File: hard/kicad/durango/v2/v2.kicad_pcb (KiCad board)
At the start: 2 copper layers, 177.8 x 130.8 mm, 155 parts, among them J1 NANOLINK, J10 STEP, J11 EXPANSION, J2 AUDIO IN, J3 IOx, J4 LED, J605 COMPONENT VIDEO, J7 POWER IN, J706 COMPOSITE, J8 DEBUG, J9 CARTRIDGE, J905 SCART, Q1 BC548, Q2 BC548, Q3 BC548, Q307 BC548, Q4 BC548, Q5 BC548, Q608 BC548, Q609 BC548, Q610 BC548, Q611 BC548, Q906 BC548, SW1 RESET, SW2 NMI, U1 65C02, U10 74HC139, U104 74HC257, U105 74HC257, U11 74HC688, U12 74HC74, U124 74HC574, U125 74HC157, U126 74HC86, U127 74HC245, U13 74HC32, U14 74HC4040, U15 74HC4040, U16 74HC02, U17 74HC21, U18 74HC85, U19 CD4040, U20 74HC85, U204 74HC257, U205 74HC257, U22 74HC175, U224 74HC166, U227 74HC20, U23 74HC86, U29 74HC139, U3 62256, U31 74HC245, U32 74HC245, U321 74HC157, U428 74HC174, U530 74HC367, U6 74HC157, U7 74HC157, U8 74HC30, U9 74HC00, X1 28 MHz

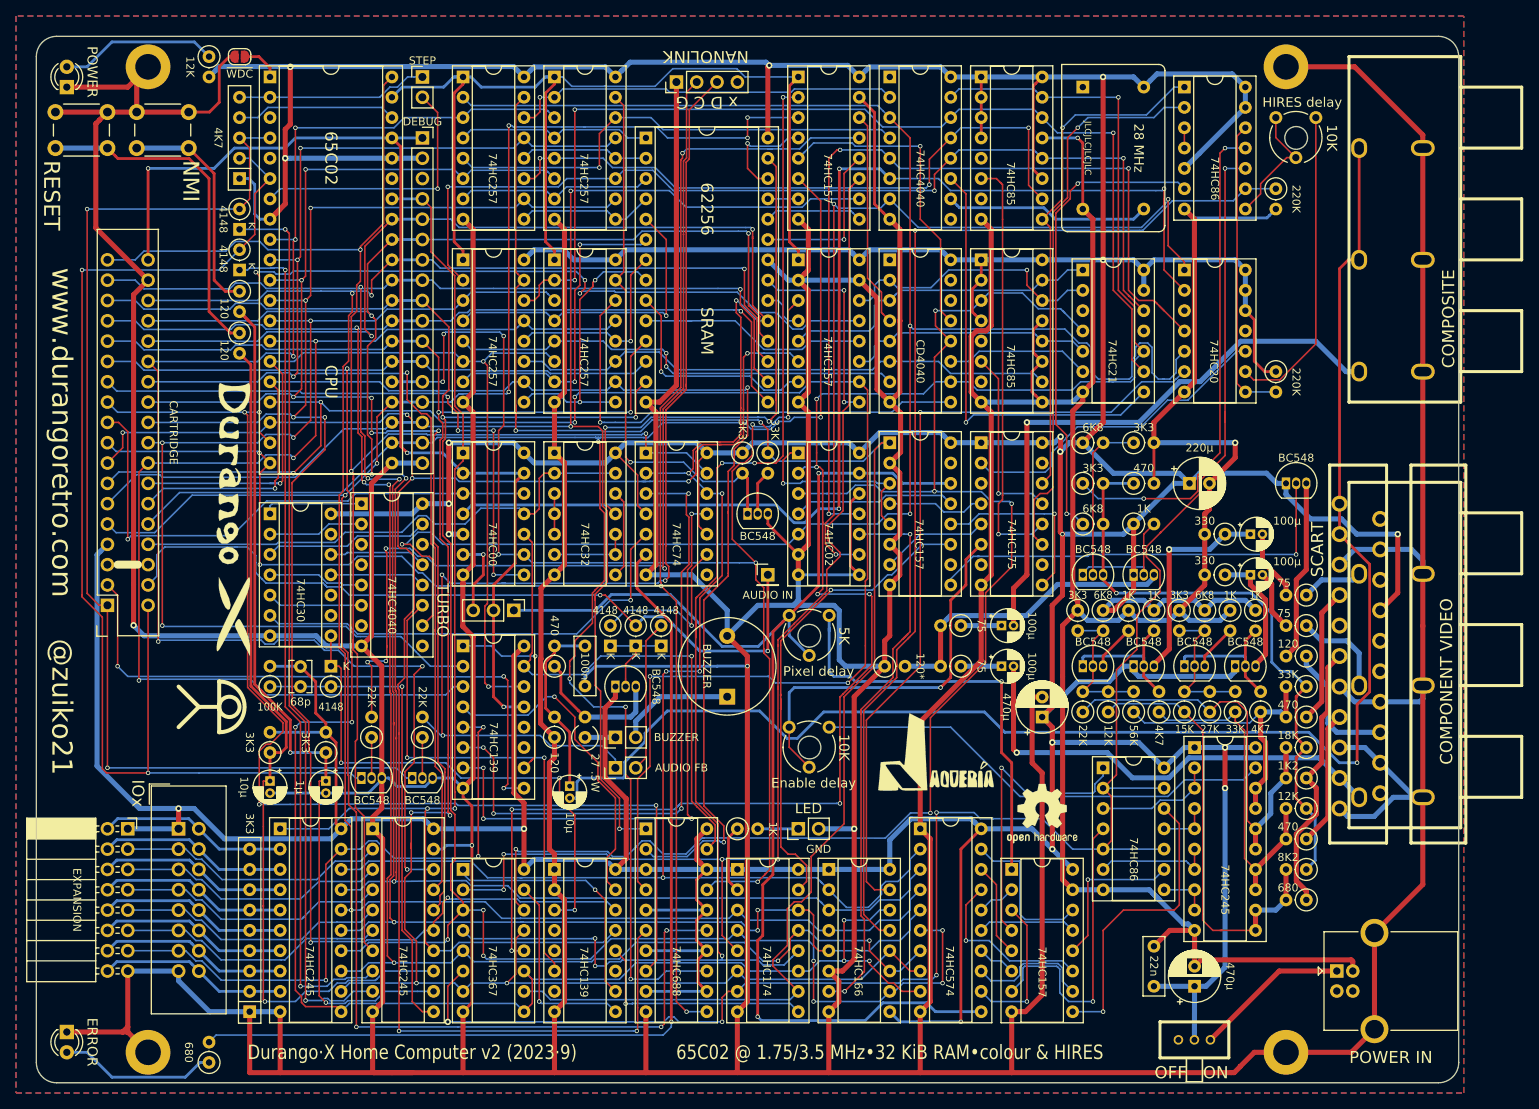
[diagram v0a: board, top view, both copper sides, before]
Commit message: mostly clean v2 PCB
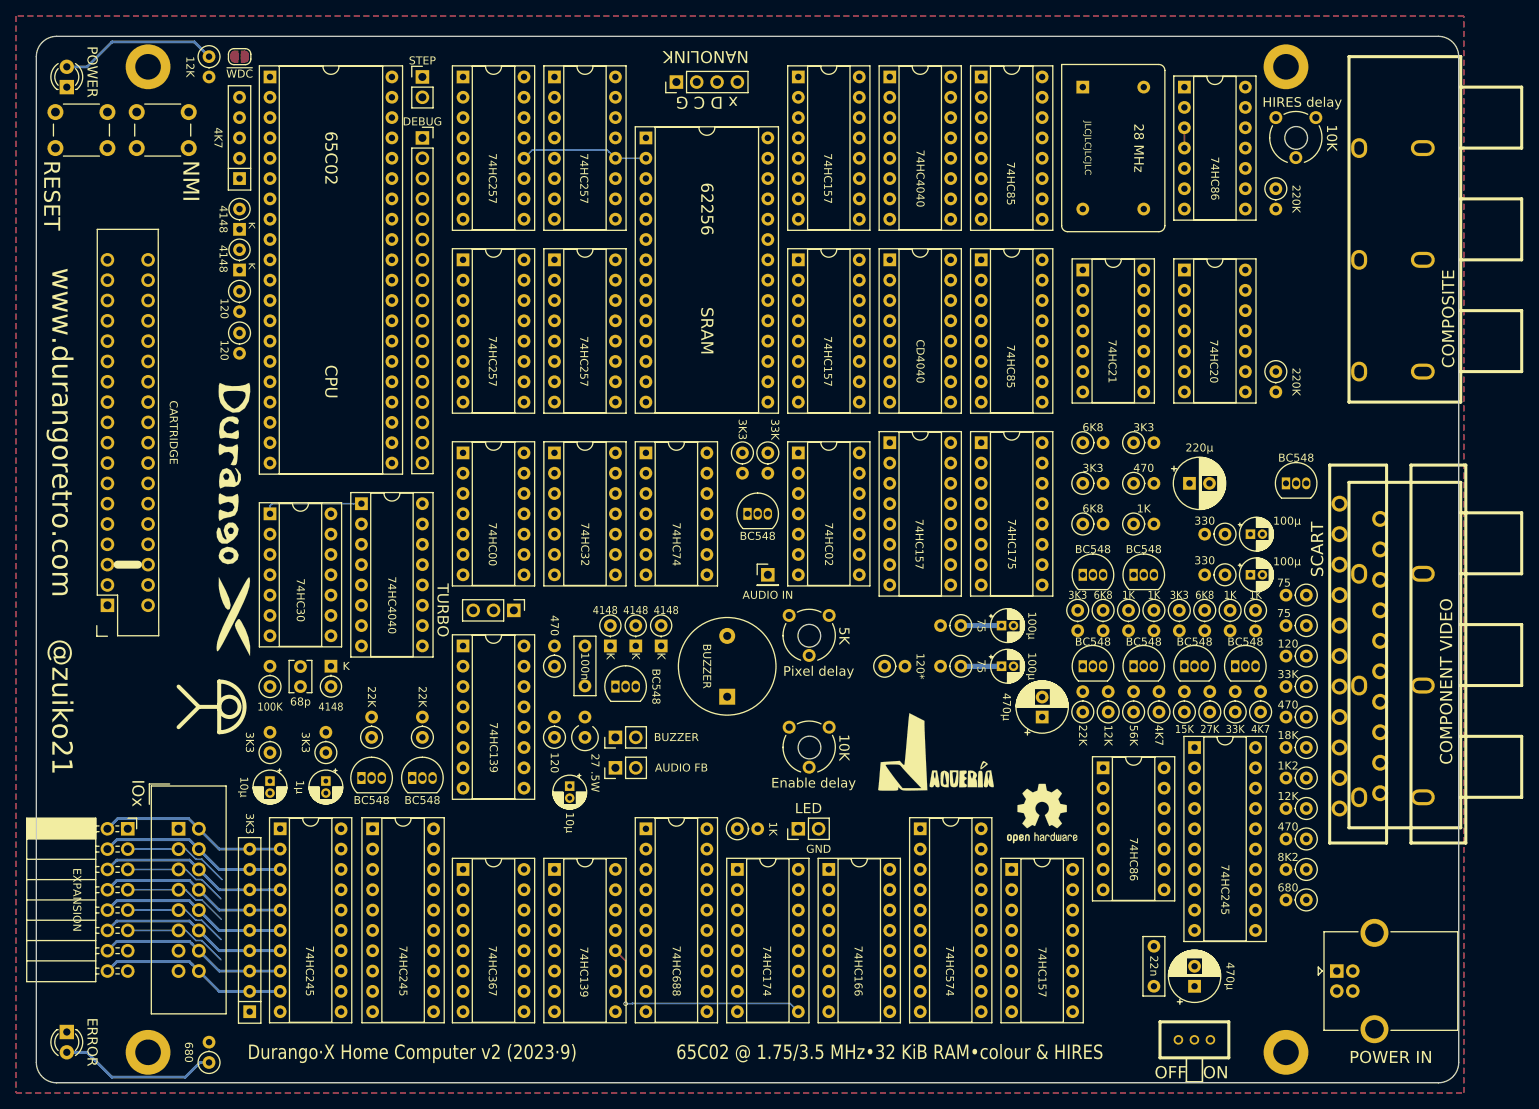
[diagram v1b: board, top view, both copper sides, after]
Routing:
- net GND: track 1762.0 -> 0.00 mm, vias 6 -> 0
- net +5V: track 1134.5 -> 0.00 mm, vias 19 -> 0
- net A2: track 595.3 -> 0.00 mm, vias 17 -> 0
- net D0: track 279.7 -> 0.00 mm, vias 8 -> 0
- net D3: track 262.5 -> 0.00 mm, vias 7 -> 0
- net D5: track 260.2 -> 0.00 mm, vias 7 -> 0
- net A14: track 257.2 -> 0.00 mm, vias 9 -> 0
- net D7: track 256.7 -> 0.00 mm, vias 6 -> 0
- net D1: track 253.7 -> 0.00 mm, vias 5 -> 0
- net D4: track 253.6 -> 0.00 mm, vias 9 -> 0
- net D2: track 248.3 -> 0.00 mm, vias 4 -> 0
- net D6: track 248.3 -> 0.00 mm, vias 6 -> 0
- net VA0: track 234.0 -> 0.00 mm, vias 3 -> 0
- net INVERT: track 229.1 -> 0.00 mm, vias 5 -> 0
- net A9: track 227.8 -> 0.00 mm, vias 7 -> 0
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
